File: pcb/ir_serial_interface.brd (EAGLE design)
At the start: 41.6 x 25.4 mm, 34 parts, among them IC1 PIC18LF2550, IC2 LP2992, T1 PS401

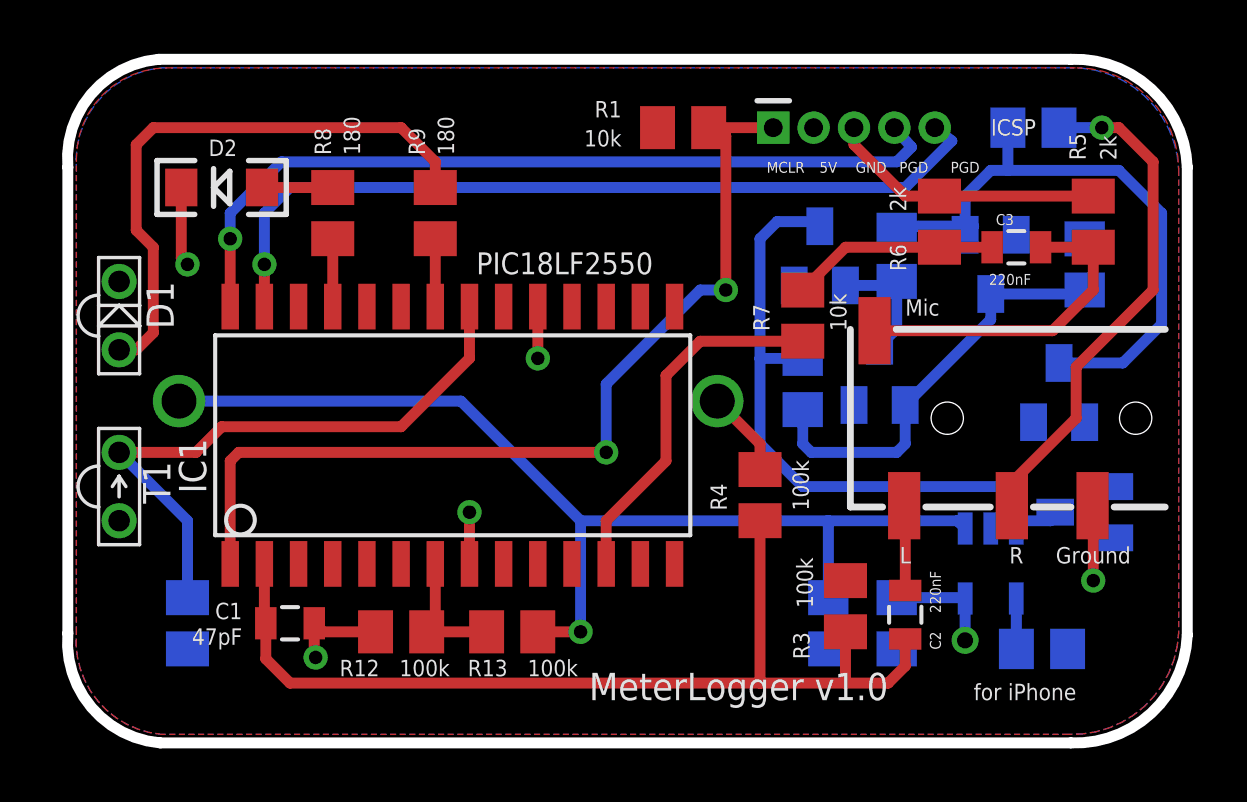
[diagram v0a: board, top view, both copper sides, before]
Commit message: PCB: final touch
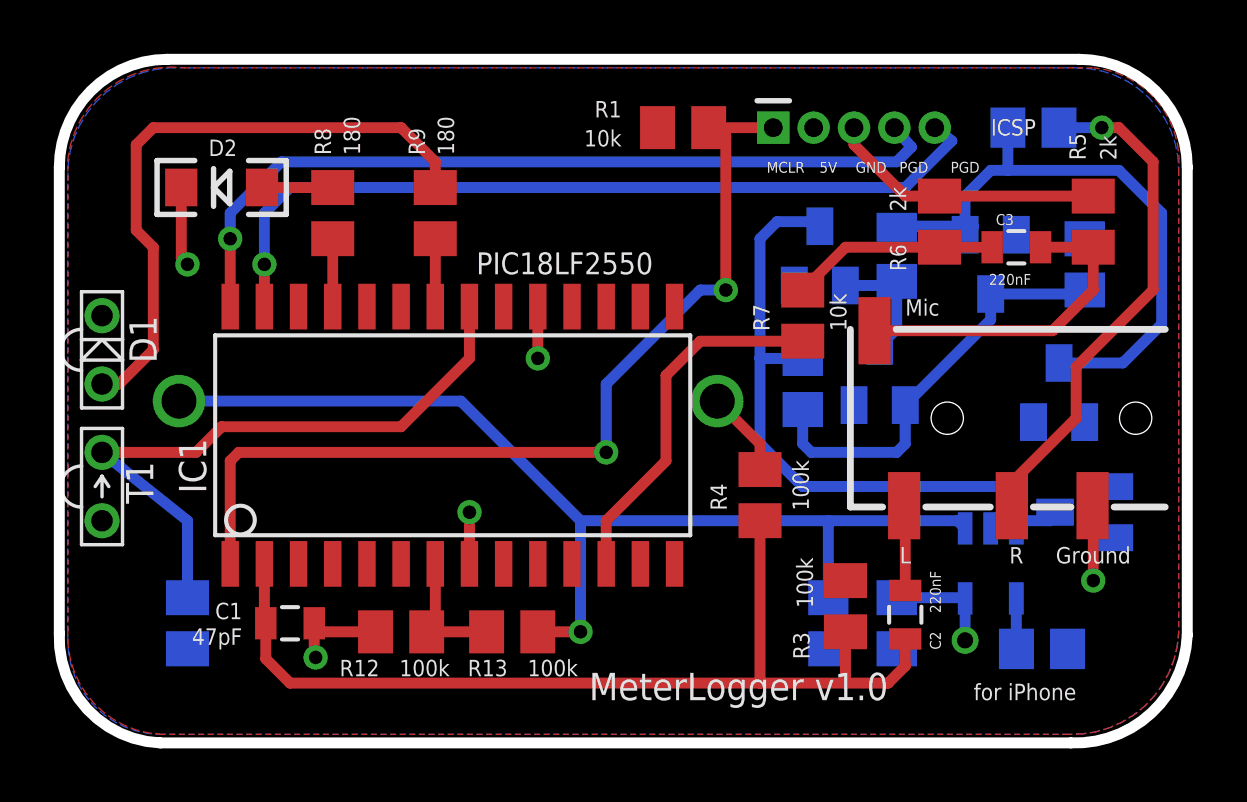
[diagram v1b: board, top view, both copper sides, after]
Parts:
- moved D1 1.42 mm to (23.5, 40.0)
- moved T1 0.63 mm to (23.5, 34.9)
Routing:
- net N$14: track 21.6 -> 23.2 mm
- net N$1: track 22.8 -> 23.9 mm
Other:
- board size 41.6 x 25.4 mm -> 41.9 x 25.4 mm
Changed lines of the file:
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@@
 <text x="50.4825" y="46.99" size="0.4064" layer="121" ratio="10" rot="R180" align="bottom-center">5V</text>
 <text x="48.895" y="46.99" size="0.4064" layer="121" ratio="10" rot="R180" align="bottom-center">MCLR</text>
-<wire x1="25.60006875" y1="50.8" x2="59.48993125" y2="50.8" width="0.4064" layer="20"/>
-<wire x1="59.48993125" y1="50.8" x2="63.8175" y2="46.78993125" width="0.4064" layer="20" curve="-90"/>
+<wire x1="25.91756875" y1="50.8" x2="59.80743125" y2="50.8" width="0.4064" layer="20"/>
+<wire x1="59.80743125" y1="50.8" x2="63.8175" y2="46.78993125" width="0.4064" layer="20" curve="-90"/>
 <wire x1="63.8175" y1="46.78993125" x2="63.8175" y2="29.41006875" width="0.4064" layer="20"/>
 <wire x1="63.8175" y1="29.41006875" x2="59.48993125" y2="25.4" width="0.4064" layer="20" curve="-90"/>
 <wire x1="59.48993125" y1="25.4" x2="25.6592875" y2="25.4" width="0.4064" layer="20"/>
-<wire x1="25.6592875" y1="25.4" x2="22.225" y2="29.4692875" width="0.4064" layer="20" curve="-90"/>
-<wire x1="22.225" y1="29.4692875" x2="22.225" y2="46.78993125" width="0.4064" layer="20"/>
-<wire x1="22.225" y1="46.78993125" x2="25.60006875" y2="50.8" width="0.4064" layer="20" curve="-90"/>
+<wire x1="25.6592875" y1="25.4" x2="21.9075" y2="29.4692875" width="0.4064" layer="20" curve="-90"/>
+<wire x1="21.9075" y1="29.4692875" x2="21.9075" y2="46.78993125" width="0.4064" layer="20"/>
+<wire x1="21.9075" y1="46.78993125" x2="25.91756875" y2="50.8" width="0.4064" layer="20" curve="-90"/>
 <text x="55.88" y="26.9875" size="0.6096" layer="121" ratio="10">for iPhone</text>
 <text x="53.34" y="32.0675" size="0.6096" layer="121" ratio="10" align="bottom-center">L</text>
@@
 </autorouter>
 <elements>
-<element name="T1" library="SparkFun-Sensors" package="LTR-301" value="PS401" x="24.13" y="34.925" smashed="yes" rot="R270">
-<attribute name="NAME" x="26.035" y="34.29" size="1.016" layer="25" ratio="10" rot="R90"/>
+<element name="T1" library="SparkFun-Sensors" package="LTR-301" value="PS401" x="23.495" y="34.925" smashed="yes" rot="R270">
+<attribute name="NAME" x="25.4" y="34.29" size="1.016" layer="25" ratio="10" rot="R90"/>
 </element>
 <element name="R2" library="resistor" package="M0805" value="10k" x="26.67" y="29.845" smashed="yes" rot="MR90">
@@
 <attribute name="VALUE" x="36.576" y="47.244" size="0.6096" layer="25" rot="R90"/>
 </element>
-<element name="D1" library="SparkFun-LED" package="LTE-302" value="IR" x="24.13" y="41.275" smashed="yes" rot="R270">
-<attribute name="NAME" x="25.146" y="42.545" size="1.016" layer="25" ratio="10" rot="R270"/>
+<element name="D1" library="SparkFun-LED" package="LTE-302" value="IR" x="23.495" y="40.005" smashed="yes" rot="R270">
+<attribute name="NAME" x="24.511" y="41.275" size="1.016" layer="25" ratio="10" rot="R270"/>
 </element>
 <element name="C8" library="rcl" package="C0805" value="220nF" x="60.0075" y="43.18" smashed="yes" rot="MR270">
@@
 <contactref element="R1" pad="1"/>
 <polygon width="0.254" layer="1" isolate="0.4064">
-<vertex x="22.5425" y="29.50980625"/>
-<vertex x="22.5425" y="47.10743125" curve="-90"/>
-<vertex x="25.91756875" y="50.4825"/>
-<vertex x="59.70769375" y="50.4825" curve="-90"/>
+<vertex x="22.225" y="29.50980625"/>
+<vertex x="22.225" y="47.10743125" curve="-90"/>
+<vertex x="26.55256875" y="50.4825"/>
+<vertex x="60.34269375" y="50.4825" curve="-90"/>
 <vertex x="63.5" y="46.69019375"/>
 <vertex x="63.5" y="29.50980625" curve="-90"/>
@@
 <contactref element="U$1" pad="3"/>
 <polygon width="0.254" layer="16" isolate="0.4064">
-<vertex x="25.69980625" y="50.4825"/>
-<vertex x="59.39019375" y="50.4825" curve="-90"/>
+<vertex x="26.01730625" y="50.4825"/>
+<vertex x="59.70769375" y="50.4825" curve="-90"/>
 <vertex x="63.5" y="46.69019375"/>
 <vertex x="63.5" y="29.50980625" curve="-90"/>
 <vertex x="59.39019375" y="25.7175"/>
 <vertex x="25.69980625" y="25.7175" curve="-90"/>
-<vertex x="22.5425" y="29.50980625"/>
-<vertex x="22.5425" y="46.69019375" curve="-90"/>
+<vertex x="22.225" y="29.19230625"/>
+<vertex x="22.225" y="46.37269375" curve="-90"/>
 </polygon>
 <contactref element="C1" pad="1"/>
@@
 <wire x1="34.6075" y1="37.1475" x2="27.94" y2="37.1475" width="0.4064" layer="1"/>
 <wire x1="27.94" y1="37.1475" x2="26.9875" y2="36.195" width="0.4064" layer="1"/>
-<wire x1="26.9875" y1="36.195" x2="24.13" y2="36.195" width="0.4064" layer="1"/>
+<wire x1="26.9875" y1="36.195" x2="23.495" y2="36.195" width="0.4064" layer="1"/>
 <wire x1="26.67" y1="30.795" x2="26.67" y2="33.655" width="0.4064" layer="16"/>
-<wire x1="26.67" y1="33.655" x2="24.13" y2="36.195" width="0.4064" layer="16"/>
+<wire x1="26.67" y1="33.655" x2="23.495" y2="36.195" width="0.4064" layer="16"/>
 </signal>
 <signal name="N$2">
@@
 <wire x1="24.765" y1="47.625" x2="24.765" y2="44.45" width="0.4064" layer="1"/>
 <wire x1="24.765" y1="44.45" x2="25.4" y2="43.815" width="0.4064" layer="1"/>
-<wire x1="25.4" y1="43.815" x2="25.4" y2="40.64" width="0.4064" layer="1"/>
-<wire x1="25.4" y1="40.64" x2="24.765" y2="40.005" width="0.4064" layer="1"/>
-<wire x1="24.765" y1="40.005" x2="24.13" y2="40.005" width="0.4064" layer="1"/>
+<wire x1="25.4" y1="43.815" x2="25.4" y2="40.005" width="0.4064" layer="1"/>
+<wire x1="25.4" y1="40.005" x2="24.13" y2="38.735" width="0.4064" layer="1"/>
+<wire x1="24.13" y1="38.735" x2="23.495" y2="38.735" width="0.4064" layer="1"/>
 </signal>
 <signal name="N$15">

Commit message: space around connectors and opto
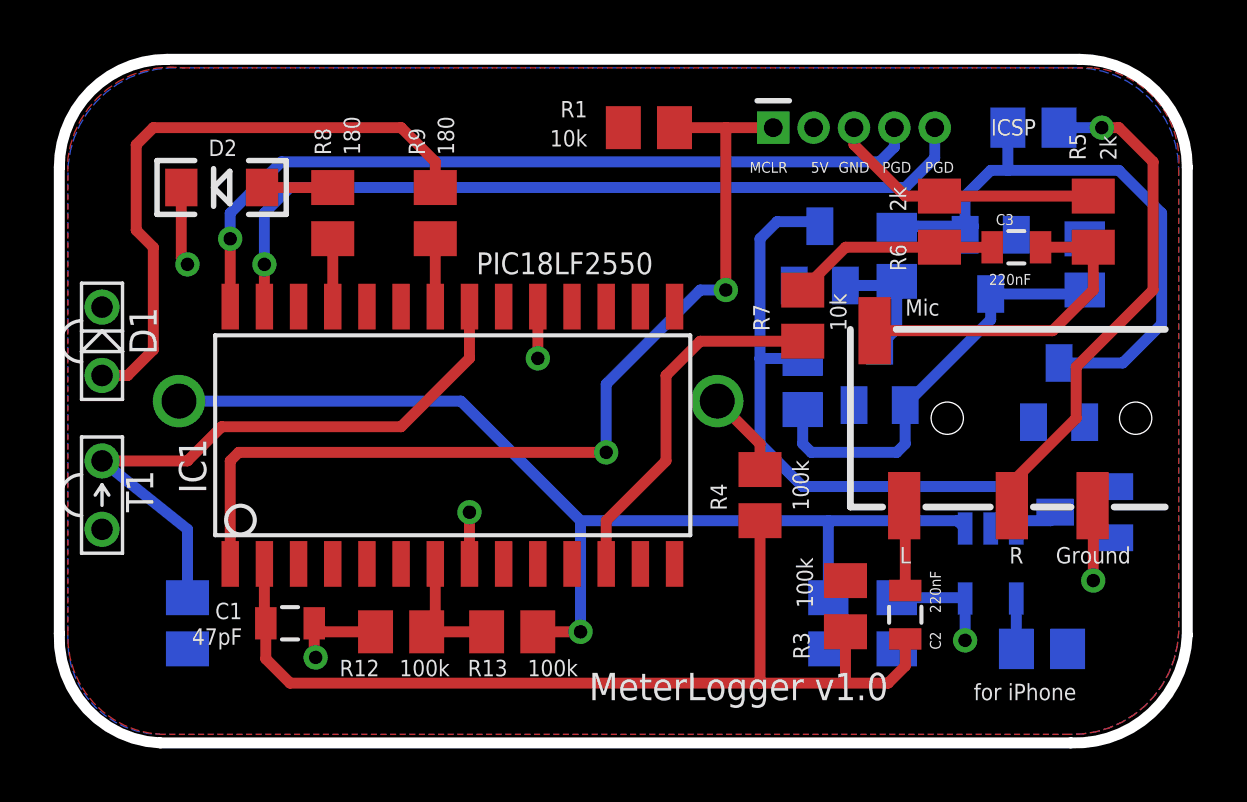
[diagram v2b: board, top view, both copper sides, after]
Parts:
- moved R1 1.27 mm to (43.8, 48.3)
- moved D1 0.32 mm to (23.5, 40.3)
- moved T1 0.32 mm to (23.5, 34.6)
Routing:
- net N$2: track 34.9 -> 36.1 mm
- net N$3: track 30.8 -> 29.9 mm
- net N$4: track 30.9 -> 30.4 mm
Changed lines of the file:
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@@
 <text x="60.0075" y="27.305" size="0.4064" layer="122" rot="MR0">(C) 2014, Kristoffer Ek + Johannes Gaardsted Jørgensen</text>
 <text x="56.515" y="48.5775" size="0.6096" layer="121" ratio="10" rot="R180" align="bottom-right">ICSP</text>
-<text x="53.6575" y="46.99" size="0.4064" layer="121" ratio="10" rot="R180" align="bottom-center">PGD</text>
-<text x="55.5625" y="46.99" size="0.4064" layer="121" ratio="10" rot="R180" align="bottom-center">PGD</text>
-<text x="52.07" y="46.99" size="0.4064" layer="121" ratio="10" rot="R180" align="bottom-center">GND</text>
-<text x="50.4825" y="46.99" size="0.4064" layer="121" ratio="10" rot="R180" align="bottom-center">5V</text>
-<text x="48.895" y="46.99" size="0.4064" layer="121" ratio="10" rot="R180" align="bottom-center">MCLR</text>
+<text x="53.0225" y="46.99" size="0.4064" layer="121" ratio="10" rot="R180" align="bottom-center">PGD</text>
+<text x="54.61" y="46.99" size="0.4064" layer="121" ratio="10" rot="R180" align="bottom-center">PGD</text>
+<text x="51.435" y="46.99" size="0.4064" layer="121" ratio="10" rot="R180" align="bottom-center">GND</text>
+<text x="50.165" y="46.99" size="0.4064" layer="121" ratio="10" rot="R180" align="bottom-center">5V</text>
+<text x="48.26" y="46.99" size="0.4064" layer="121" ratio="10" rot="R180" align="bottom-center">MCLR</text>
 <wire x1="25.91756875" y1="50.8" x2="59.80743125" y2="50.8" width="0.4064" layer="20"/>
 <wire x1="59.80743125" y1="50.8" x2="63.8175" y2="46.78993125" width="0.4064" layer="20" curve="-90"/>
@@
 </autorouter>
 <elements>
-<element name="T1" library="SparkFun-Sensors" package="LTR-301" value="PS401" x="23.495" y="34.925" smashed="yes" rot="R270">
-<attribute name="NAME" x="25.4" y="34.29" size="1.016" layer="25" ratio="10" rot="R90"/>
+<element name="T1" library="SparkFun-Sensors" package="LTR-301" value="PS401" x="23.495" y="34.6075" smashed="yes" rot="R270">
+<attribute name="NAME" x="25.4" y="33.9725" size="1.016" layer="25" ratio="10" rot="R90"/>
 </element>
 <element name="R2" library="resistor" package="M0805" value="10k" x="26.67" y="29.845" smashed="yes" rot="MR90">
@@
 </element>
 <element name="U$1" library="SparkFun-Connectors" package="PIC-ICSP-MINI" value="PIC-ICSP-MINI" x="51.435" y="48.26"/>
-<element name="R1" library="resistor" package="M0805" value="10k" x="45.085" y="48.26" smashed="yes">
-<attribute name="NAME" x="42.799" y="48.641" size="0.6096" layer="25" align="bottom-right"/>
-<attribute name="VALUE" x="42.799" y="47.5615" size="0.6096" layer="25" align="bottom-right"/>
+<element name="R1" library="resistor" package="M0805" value="10k" x="43.815" y="48.26" smashed="yes">
+<attribute name="NAME" x="41.529" y="48.641" size="0.6096" layer="25" align="bottom-right"/>
+<attribute name="VALUE" x="41.529" y="47.5615" size="0.6096" layer="25" align="bottom-right"/>
 </element>
 <element name="R3" library="resistor" package="M0805" value="100k" x="51.1175" y="30.48" smashed="yes" rot="R90">
@@
 <attribute name="VALUE" x="36.576" y="47.244" size="0.6096" layer="25" rot="R90"/>
 </element>
-<element name="D1" library="SparkFun-LED" package="LTE-302" value="IR" x="23.495" y="40.005" smashed="yes" rot="R270">
-<attribute name="NAME" x="24.511" y="41.275" size="1.016" layer="25" ratio="10" rot="R270"/>
+<element name="D1" library="SparkFun-LED" package="LTE-302" value="IR" x="23.495" y="40.3225" smashed="yes" rot="R270">
+<attribute name="NAME" x="24.511" y="41.5925" size="1.016" layer="25" ratio="10" rot="R270"/>
 </element>
 <element name="C8" library="rcl" package="C0805" value="220nF" x="60.0075" y="43.18" smashed="yes" rot="MR270">
@@
 <wire x1="55.565" y1="30.7675" x2="55.565" y2="29.2125" width="0.4064" layer="16"/>
 <wire x1="55.565" y1="29.2125" x2="55.5625" y2="29.21" width="0.4064" layer="16"/>
-<via x="55.5625" y="29.21" extent="1-16" drill="0.6"/>
+<via x="55.5625" y="29.21" extent="1-16" drill="0.5"/>
 <contactref element="C5" pad="1"/>
 <wire x1="53.0225" y1="30.795" x2="55.5375" y2="30.795" width="0.4064" layer="16"/>
@@
 <wire x1="37.1475" y1="39.6875" x2="34.6075" y2="37.1475" width="0.4064" layer="1"/>
 <wire x1="34.6075" y1="37.1475" x2="27.94" y2="37.1475" width="0.4064" layer="1"/>
-<wire x1="27.94" y1="37.1475" x2="26.9875" y2="36.195" width="0.4064" layer="1"/>
-<wire x1="26.9875" y1="36.195" x2="23.495" y2="36.195" width="0.4064" layer="1"/>
-<wire x1="26.67" y1="30.795" x2="26.67" y2="33.655" width="0.4064" layer="16"/>
-<wire x1="26.67" y1="33.655" x2="23.495" y2="36.195" width="0.4064" layer="16"/>
+<wire x1="26.67" y1="30.795" x2="26.67" y2="33.3375" width="0.4064" layer="16"/>
+<wire x1="26.67" y1="33.3375" x2="23.495" y2="35.8775" width="0.4064" layer="16"/>
+<wire x1="27.94" y1="37.1475" x2="26.67" y2="35.8775" width="0.4064" layer="1"/>
+<wire x1="26.67" y1="35.8775" x2="23.495" y2="35.8775" width="0.4064" layer="1"/>
 </signal>
 <signal name="N$2">
@@
 <contactref element="R1" pad="2"/>
 <contactref element="IC1" pad="1"/>
-<wire x1="48.435" y1="48.26" x2="46.355" y2="48.26" width="0.4064" layer="1"/>
-<wire x1="46.355" y1="48.26" x2="46.035" y2="48.26" width="0.4064" layer="1"/>
+<wire x1="48.435" y1="48.26" x2="46.6725" y2="48.26" width="0.4064" layer="1"/>
+<wire x1="46.6725" y1="48.26" x2="44.765" y2="48.26" width="0.4064" layer="1"/>
 <via x="42.2275" y="36.195" extent="1-16" drill="0.5"/>
 <via x="46.6725" y="42.2275" extent="1-16" drill="0.5"/>
@@
 <wire x1="28.2575" y1="35.8775" x2="28.575" y2="36.195" width="0.4064" layer="1"/>
 <wire x1="28.575" y1="36.195" x2="42.2275" y2="36.195" width="0.4064" layer="1"/>
-<wire x1="46.6725" y1="42.2275" x2="46.6725" y2="47.9425" width="0.4064" layer="1"/>
-<wire x1="46.6725" y1="47.9425" x2="46.355" y2="48.26" width="0.4064" layer="1"/>
+<wire x1="46.6725" y1="42.2275" x2="46.6725" y2="48.26" width="0.4064" layer="1"/>
 <wire x1="46.6725" y1="42.2275" x2="45.72" y2="42.2275" width="0.4064" layer="16"/>
 <wire x1="45.72" y1="42.2275" x2="42.2275" y2="38.735" width="0.4064" layer="16"/>
@@
 <contactref element="U$1" pad="4"/>
 <contactref element="IC1" pad="28"/>
-<wire x1="52.935" y1="48.26" x2="53.57" y2="47.5375" width="0.4064" layer="16"/>
-<wire x1="53.57" y1="47.5375" x2="53.0225" y2="46.99" width="0.4064" layer="16"/>
-<wire x1="53.0225" y1="46.99" x2="30.1625" y2="46.99" width="0.4064" layer="16"/>
+<wire x1="52.935" y1="48.26" x2="52.935" y2="47.5375" width="0.4064" layer="16"/>
+<wire x1="52.935" y1="47.5375" x2="52.3875" y2="46.99" width="0.4064" layer="16"/>
+<wire x1="52.3875" y1="46.99" x2="30.1625" y2="46.99" width="0.4064" layer="16"/>
 <wire x1="30.1625" y1="46.99" x2="28.2575" y2="45.085" width="0.4064" layer="16"/>
 <wire x1="28.2575" y1="45.085" x2="28.2575" y2="44.1325" width="0.4064" layer="16"/>
@@
 <contactref element="U$1" pad="5"/>
 <contactref element="IC1" pad="27"/>
-<wire x1="54.435" y1="48.26" x2="55.07" y2="47.7675" width="0.4064" layer="16"/>
-<wire x1="55.07" y1="47.7675" x2="53.34" y2="46.0375" width="0.4064" layer="16"/>
+<wire x1="54.435" y1="48.26" x2="54.435" y2="47.1325" width="0.4064" layer="16"/>
+<wire x1="54.435" y1="47.1325" x2="53.34" y2="46.0375" width="0.4064" layer="16"/>
 <via x="29.5275" y="43.18" extent="1-16" drill="0.5"/>
 <wire x1="29.5275" y1="43.18" x2="29.5275" y2="41.61" width="0.4064" layer="1"/>
@@
 <wire x1="24.765" y1="44.45" x2="25.4" y2="43.815" width="0.4064" layer="1"/>
 <wire x1="25.4" y1="43.815" x2="25.4" y2="40.005" width="0.4064" layer="1"/>
-<wire x1="25.4" y1="40.005" x2="24.13" y2="38.735" width="0.4064" layer="1"/>
-<wire x1="24.13" y1="38.735" x2="23.495" y2="38.735" width="0.4064" layer="1"/>
+<wire x1="25.4" y1="40.005" x2="24.4475" y2="39.0525" width="0.4064" layer="1"/>
+<wire x1="24.4475" y1="39.0525" x2="23.495" y2="39.0525" width="0.4064" layer="1"/>
 </signal>
 <signal name="N$15">
